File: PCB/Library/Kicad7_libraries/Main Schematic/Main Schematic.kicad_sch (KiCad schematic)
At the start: 0 parts

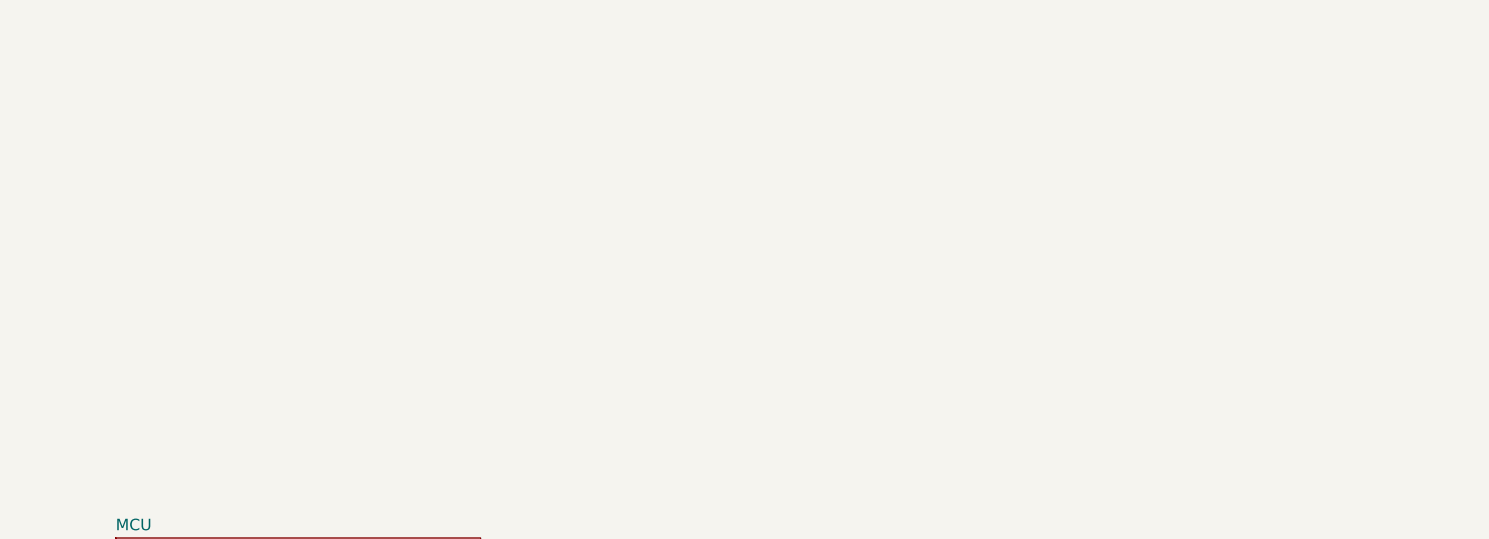
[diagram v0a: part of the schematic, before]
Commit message: updated sche
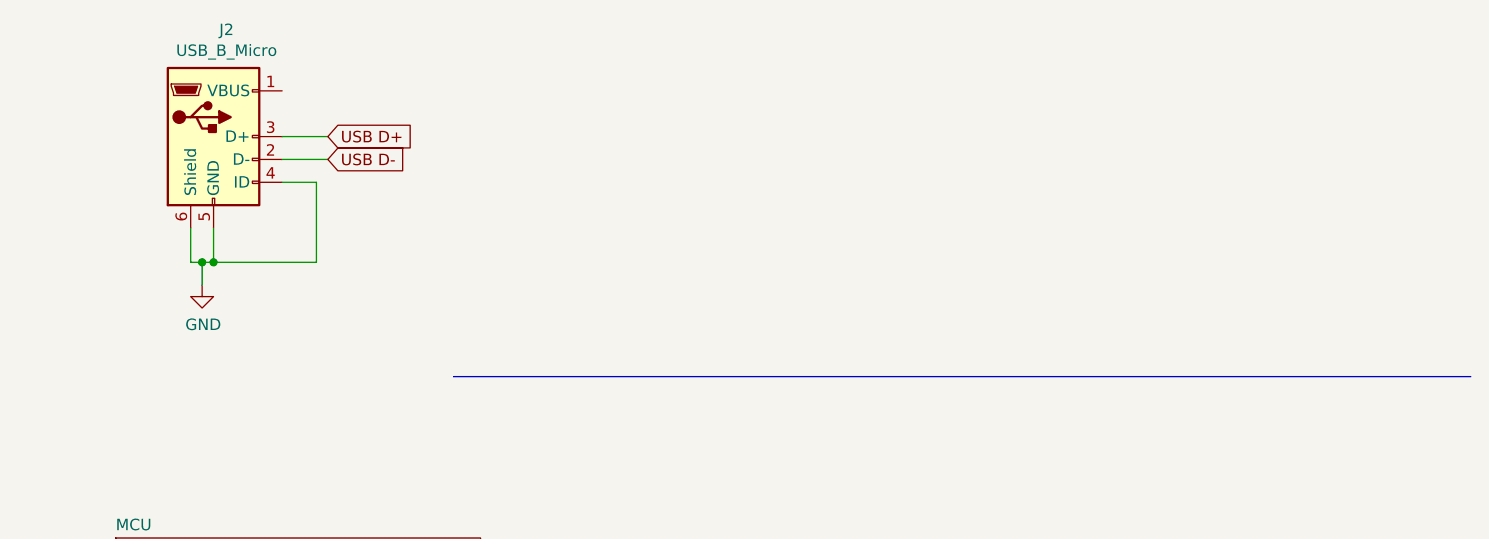
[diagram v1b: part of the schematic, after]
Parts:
- added J2: USB_B_Micro, symbol Connector:USB_B_Micro
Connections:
- new net GND: J2.4 (ID), J2.5 (GND), J2.6 (Shield)
- new net USB D+: J2.3 (D+)
- new net USB D-: J2.2 (D-)
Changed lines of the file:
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@@
 (kicad_sch (version 20230121) (generator eeschema)
   (paper "A4")
+  (junction (at 142.24 58.42) (diameter 0) (color 0 0 0 0)
+  )
+  (junction (at 140.97 58.42) (diameter 0) (color 0 0 0 0)
+  )
+  (wire (pts (xy 149.86 44.45) (xy 154.94 44.45))
+    (stroke (width 0) (type default))
+  )
+  (wire (pts (xy 153.67 58.42) (xy 142.24 58.42))
+    (stroke (width 0) (type default))
+  )
+  (wire (pts (xy 149.86 49.53) (xy 153.67 49.53))
+    (stroke (width 0) (type default))
+  )
+  (wire (pts (xy 153.67 49.53) (xy 153.67 58.42))
+    (stroke (width 0) (type default))
+  )
+  (wire (pts (xy 149.86 46.99) (xy 154.94 46.99))
+    (stroke (width 0) (type default))
+  )
+  (polyline (pts (xy 168.91 71.12) (xy 281.94 71.12))
+    (stroke (width 0) (type default))
+  )
+  (wire (pts (xy 140.97 60.96) (xy 140.97 58.42))
+    (stroke (width 0) (type default))
+  )
+  (wire (pts (xy 140.97 58.42) (xy 142.24 58.42))
+    (stroke (width 0) (type default))
+  )
+  (wire (pts (xy 140.97 58.42) (xy 139.7 58.42))
+    (stroke (width 0) (type default))
+  )
+  (wire (pts (xy 142.24 58.42) (xy 142.24 54.61))
+    (stroke (width 0) (type default))
+  )
+  (wire (pts (xy 139.7 58.42) (xy 139.7 54.61))
+    (stroke (width 0) (type default))
+  )
+  (global_label "USB D+" (shape input) (at 154.94 44.45 0) (fields_autoplaced)
+    (effects (font (size 1.27 1.27)) (justify left))
+    (property "Intersheetrefs" "${INTERSHEET_REFS}" (at 165.2602 44.45 0)
+      (effects (font (size 1.27 1.27)) (justify left) hide)
+    )
+  )
+  (global_label "USB D-" (shape input) (at 154.94 46.99 0) (fields_autoplaced)
+    (effects (font (size 1.27 1.27)) (justify left))
+    (property "Intersheetrefs" "${INTERSHEET_REFS}" (at 165.2602 46.99 0)
+      (effects (font (size 1.27 1.27)) (justify left) hide)
+    )
+  )
   (hierarchical_label "SCL" (shape input) (at 131.5212 100.6856 0) (fields_autoplaced)
     (effects (font (size 1.27 1.27)) (justify left))
@@
     (effects (font (size 1.27 1.27)) (justify left))
   )
+  (symbol (lib_id "Connector:USB_B_Micro") (at 142.24 44.45 0) (unit 1)
+    (in_bom yes) (on_board yes) (dnp no)
+    (property "Reference" "J2" (at 143.6878 32.5882 0)
+      (effects (font (size 1.27 1.27)))
+    )
+    (property "Value" "USB_B_Micro" (at 143.6878 34.8996 0)
+      (effects (font (size 1.27 1.27)))
+    )
+    (property "Footprint" "" (at 146.05 45.72 0)
+      (effects (font (size 1.27 1.27)) hide)
+    )
+    (property "Datasheet" "~" (at 146.05 45.72 0)
+      (effects (font (size 1.27 1.27)) hide)
+    )
+    (pin "1")
+    (pin "2")
+    (pin "3")
+    (pin "4")
+    (pin "5")
+    (pin "6")
+    (instances
+      (project "Main Schematic"
+        (path "/7e8c9ffe-1b32-4326-ae61-8877b5395b8a/98e117a5-3aeb-416f-98c5-160b7cf15fec"
+          (reference "J2") (unit 1)
+        )
+      )
+      (project "Main Schematic"
+        (path "/81c41bad-bb43-41af-b405-18d135a809b1/be77d6c5-6f74-462b-ad7c-0ffad190e576"
+          (reference "J2") (unit 1)
+        )
+        (path "/81c41bad-bb43-41af-b405-18d135a809b1"
+          (reference "J3") (unit 1)
+        )
+      )
+      (project "PowerUnit_sch"
+        (path "/94a75581-cd2d-4b84-bb57-dd404d2f6711"
+          (reference "J2") (unit 1)
+        )
+      )
+      (project "power supplly[2803]"
+        (path "/ef6f5e70-2168-4df2-b1ca-c7d9a0d51980"
+          (reference "J2") (unit 1)
+        )
+      )
+    )
+  )
+  (symbol (lib_id "power:GND") (at 140.97 60.96 0) (unit 1)
+    (in_bom yes) (on_board yes) (dnp no)
+    (property "Reference" "#PWR015" (at 140.97 67.31 0)
+      (effects (font (size 1.27 1.27)) hide)
+    )
+    (property "Value" "GND" (at 141.097 65.3542 0)
+      (effects (font (size 1.27 1.27)))
+    )
+    (property "Footprint" "" (at 140.97 60.96 0)
+      (effects (font (size 1.27 1.27)) hide)
+    )
+    (property "Datasheet" "" (at 140.97 60.96 0)
+      (effects (font (size 1.27 1.27)) hide)
+    )
+    (pin "1")
+    (instances
+      (project "Main Schematic"
+        (path "/7e8c9ffe-1b32-4326-ae61-8877b5395b8a/98e117a5-3aeb-416f-98c5-160b7cf15fec"
+          (reference "#PWR015") (unit 1)
+        )
+      )
+      (project "Main Schematic"
+        (path "/81c41bad-bb43-41af-b405-18d135a809b1/be77d6c5-6f74-462b-ad7c-0ffad190e576"
+          (reference "#PWR013") (unit 1)
+        )
+        (path "/81c41bad-bb43-41af-b405-18d135a809b1"
+          (reference "#PWR012") (unit 1)
+        )
+      )
+      (project "PowerUnit_sch"
+        (path "/94a75581-cd2d-4b84-bb57-dd404d2f6711"
+          (reference "#PWR015") (unit 1)
+        )
+      )
+      (project "power supplly[2803]"
+        (path "/ef6f5e70-2168-4df2-b1ca-c7d9a0d51980"
+          (reference "#PWR0105") (unit 1)
+        )
+      )
+    )
+  )
   (sheet (at 131.3688 89.0524) (size 40.5384 28.5496) (fields_autoplaced)
